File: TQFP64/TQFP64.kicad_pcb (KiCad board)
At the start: 2 copper layers, 81.5 x 20.6 mm, 12 parts, among them J1 Conn_01x32, J2 Conn_02x32_Counter_Clockwise, J3 Conn_02x32_Counter_Clockwise, J4 Conn_02x32_Counter_Clockwise, J5 Conn_01x32, J6 Conn_01x06

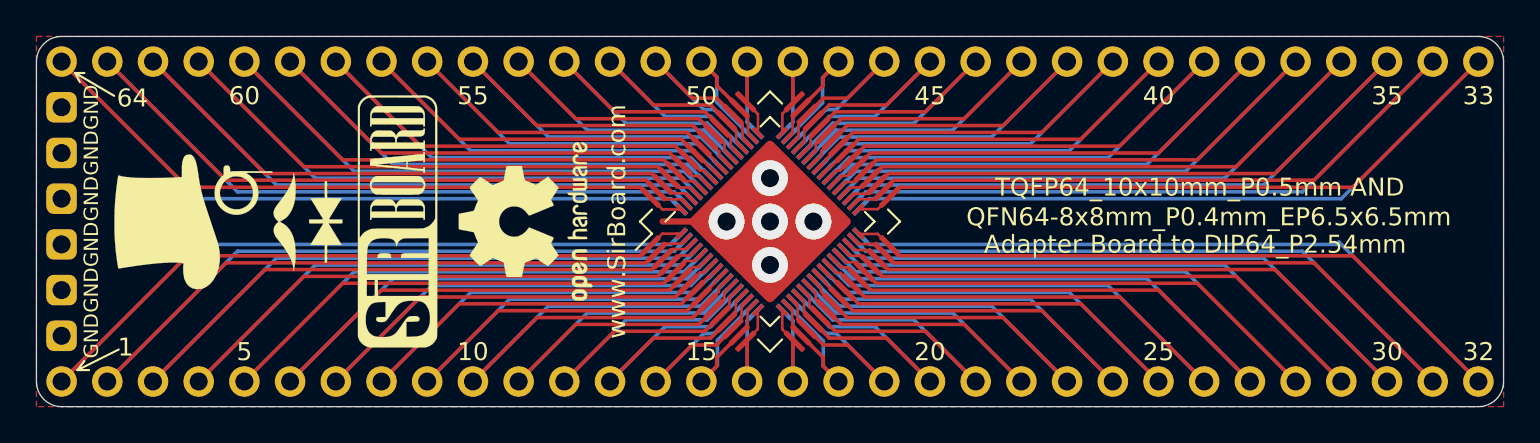
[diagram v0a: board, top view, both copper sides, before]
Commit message: Board Updates
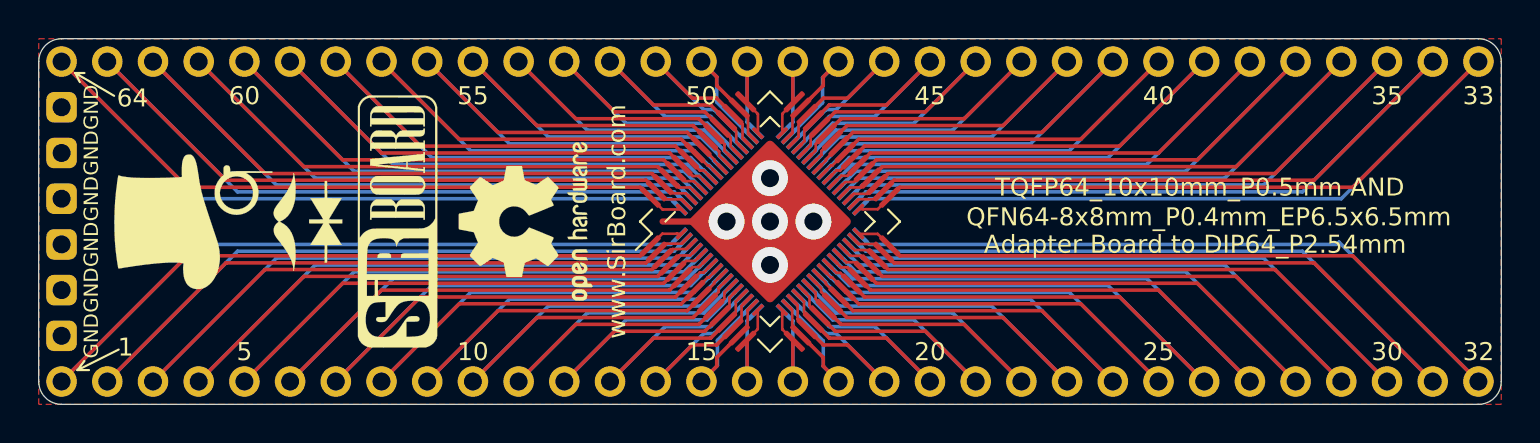
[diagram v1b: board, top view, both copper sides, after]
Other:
- board size 81.5 x 20.6 mm -> 81.3 x 20.3 mm
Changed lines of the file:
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@@
     (35 F.Paste user hide)
     (36 B.SilkS user)
-    (37 F.SilkS user hide)
+    (37 F.SilkS user)
     (38 B.Mask user hide)
     (39 F.Mask user hide)
@@
     )
   )
+  (gr_line (start 108.966 43.942) (end 108.966 26.162) (layer Edge.Cuts) (width 0.05))
+  (gr_line (start 28.956 45.212) (end 107.696 45.212) (layer Edge.Cuts) (width 0.05))
+  (gr_line (start 27.686 26.162) (end 27.686 43.942) (layer Edge.Cuts) (width 0.05))
+  (gr_line (start 107.696 24.892) (end 28.956 24.892) (layer Edge.Cuts) (width 0.05))
+  (gr_arc (start 107.696 26.162) (end 108.966 26.162) (angle -90) (layer Edge.Cuts) (width 0.05))
+  (gr_arc (start 107.696 43.942) (end 107.696 45.212) (angle -90) (layer Edge.Cuts) (width 0.05))
+  (gr_arc (start 28.956 43.942) (end 27.686 43.942) (angle -90) (layer Edge.Cuts) (width 0.05))
+  (gr_arc (start 28.956 26.162) (end 28.956 24.892) (angle -90) (layer Edge.Cuts) (width 0.05))
   (gr_text "Adapter Board to DIP64_P2.54mm" (at 91.821 34.163 180) (layer B.SilkS)
     (effects (font (size 1 1) (thickness 0.15)) (justify mirror))
@@
     (arrow2b (pts (xy 27.559 19.939) (xy 28.685504 19.352579)))
   )
-  (gr_line (start 109.093 43.942) (end 109.093 26.162) (layer Edge.Cuts) (width 0.05))
-  (gr_line (start 28.956 45.339) (end 107.696 45.339) (layer Edge.Cuts) (width 0.05))
-  (gr_line (start 27.559 26.162) (end 27.559 43.942) (layer Edge.Cuts) (width 0.05))
-  (gr_line (start 107.696 24.765) (end 28.956 24.765) (layer Edge.Cuts) (width 0.05))
-  (gr_arc (start 107.696 26.162) (end 109.093 26.162) (angle -90) (layer Edge.Cuts) (width 0.05))
-  (gr_arc (start 107.696 43.942) (end 107.696 45.339) (angle -90) (layer Edge.Cuts) (width 0.05))
-  (gr_arc (start 28.956 43.942) (end 27.559 43.942) (angle -90) (layer Edge.Cuts) (width 0.05))
-  (gr_arc (start 28.956 26.162) (end 28.956 24.765) (angle -90) (layer Edge.Cuts) (width 0.05))
   (dimension 17.78 (width 0.12) (layer Dwgs.User)
     (gr_text "17.780 mm" (at 24.384 35.052 90) (layer Dwgs.User)
@@
     (polygon
       (pts
-        (xy 27.559 24.765) (xy 109.093 24.765) (xy 109.093 45.339) (xy 27.559 45.339)
+        (xy 27.686 24.892) (xy 108.966 24.892) (xy 108.966 45.212) (xy 27.686 45.212)
       )
     )
